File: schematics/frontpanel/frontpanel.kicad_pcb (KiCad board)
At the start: 2 copper layers, 72.4 x 21.6 mm, 10 parts, among them J1 Conn_01x02_Male, J2 Conn_01x02_Male, J3 Conn_01x03_Male, J4 Conn_01x03_Male, SW1 SW_Push, SW2 SW_Push

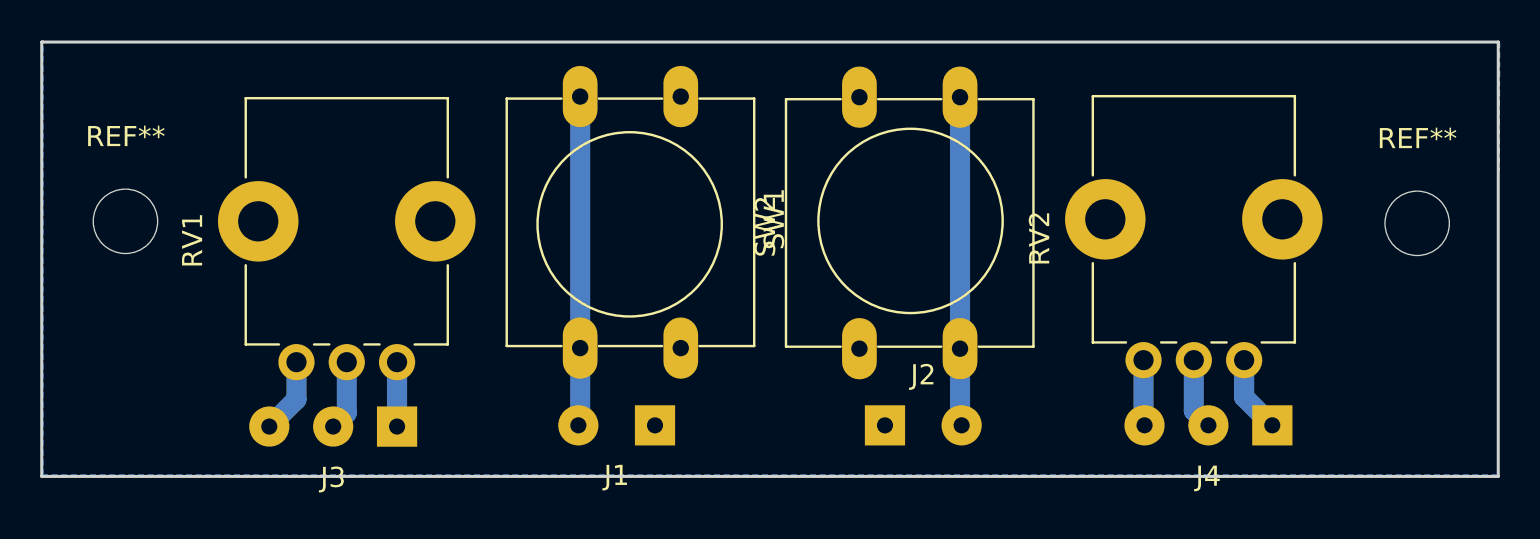
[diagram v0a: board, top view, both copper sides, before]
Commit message: Updated PCB image files
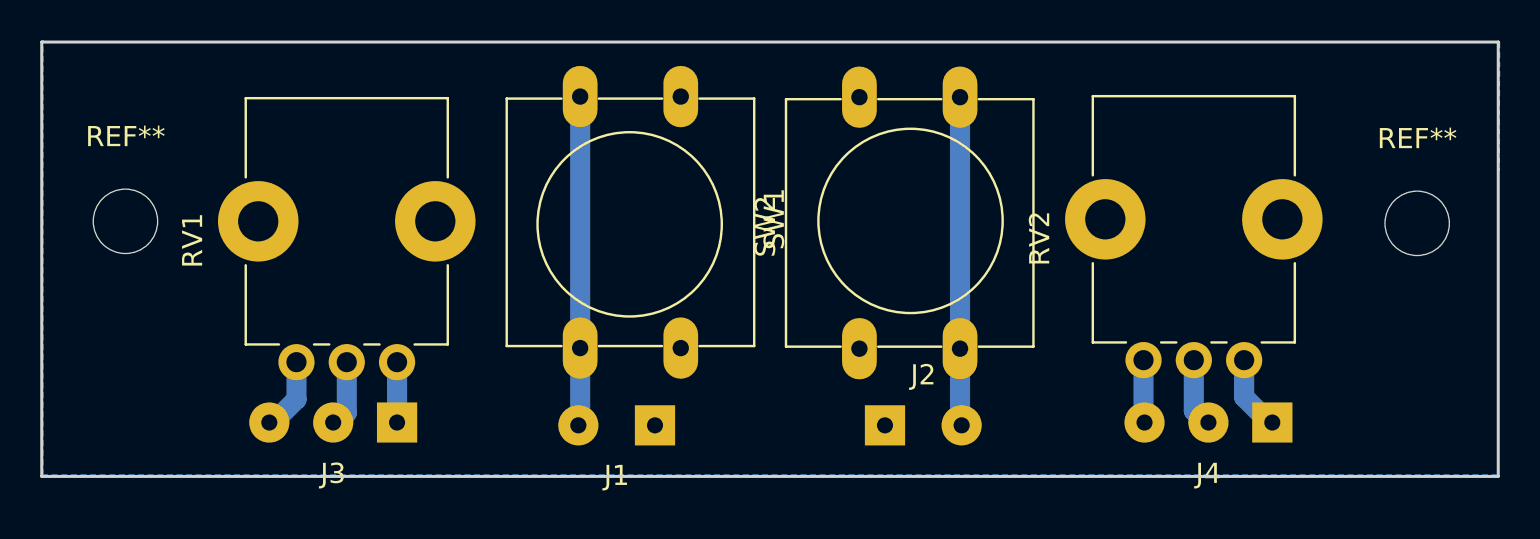
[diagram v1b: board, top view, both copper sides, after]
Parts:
- moved J3 0.20 mm to (58.3, 129.4)
- moved J4 0.14 mm to (101.8, 129.4)
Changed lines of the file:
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@@
       (outputformat 5)
       (mirror false)
-      (drillshape 2)
+      (drillshape 1)
       (scaleselection 1)
       (outputdirectory ""))
@@
   )
   (module Connector_Wire:SolderWirePad_1x03_P3.175mm_Drill0.8mm (layer F.Cu)
-    (at 58.3 129.6 180)
+    (at 58.3 129.4 180)
     (descr "Wire solder connection")
     (tags connector)
@@
   )
   (module Connector_Wire:SolderWirePad_1x03_P3.175mm_Drill0.8mm (layer F.Cu)
-    (at 101.8 129.54 180)
+    (at 101.8 129.4 180)
     (descr "Wire solder connection")
     (tags connector)
